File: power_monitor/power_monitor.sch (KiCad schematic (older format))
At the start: 8 parts, among them J1 230V AC Input, J2 230V AC Output, J3 RFID, J4 OLED, J5 WS2812, U1 Wemos-D1-mini

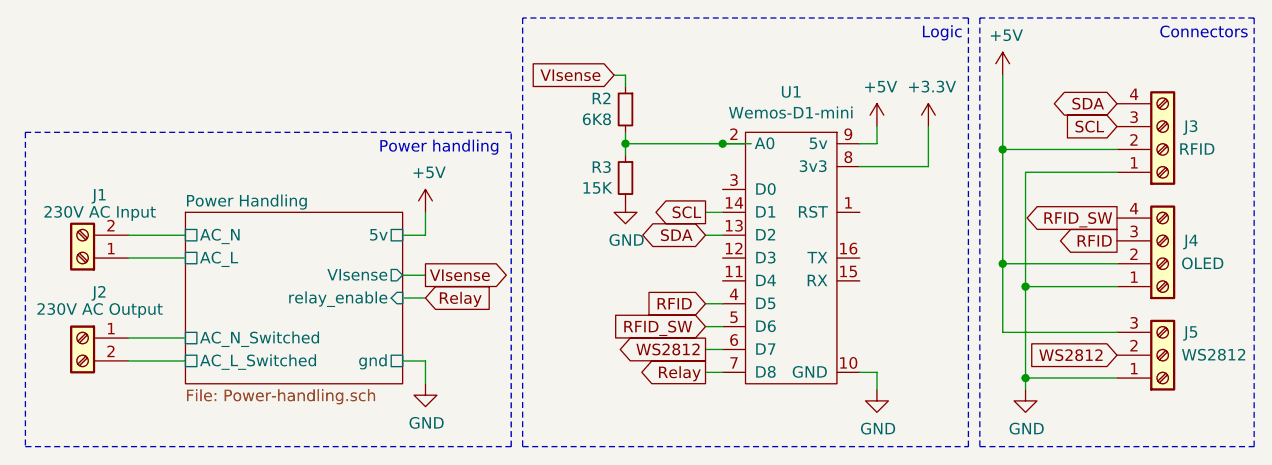
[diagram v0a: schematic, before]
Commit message: Added gerbers
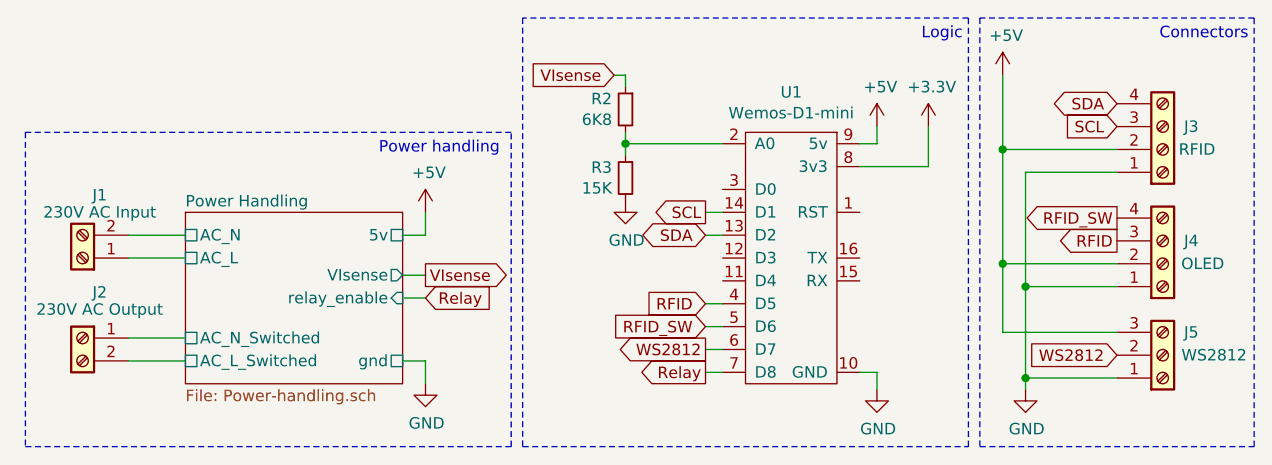
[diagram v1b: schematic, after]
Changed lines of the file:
@@
 Wire Wire Line
 	5600 3100 5600 3150
-Wire Wire Line
-	5600 3350 5600 3400
-Wire Wire Line
-	5600 3400 6025 3400
 $Comp
 L Device:R_Small R3
@@
 	-1   0    0    -1
 $EndComp
-Wire Wire Line
-	5600 3400 5600 3450
-Connection ~ 5600 3400
 $Comp
 L power:GND #PWR0109
@@
 Wire Notes Line
 	5150 4725 7100 4725
-Connection ~ 6025 3400
-Wire Wire Line
-	6025 3400 6150 3400
 Text Notes 8325 2950 2    50   ~ 0
 Connectors
@@
 Text Notes 5050 3450 2    50   ~ 0
 Power handling
+Wire Wire Line
+	5600 3350 5600 3400
+Wire Wire Line
+	6025 3400 5600 3400
+Connection ~ 5600 3400
+Wire Wire Line
+	5600 3400 5600 3450
 $EndSCHEMATC
